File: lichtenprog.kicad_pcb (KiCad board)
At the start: 2 copper layers, 29 x 34 mm, 34 parts, among them J1 USB_B_Mini, J2 Conn_01x08, U1 AMS1117-3.3, U2 CP2102N-A01-GQFN28, U3 MCP6L04x-xSL

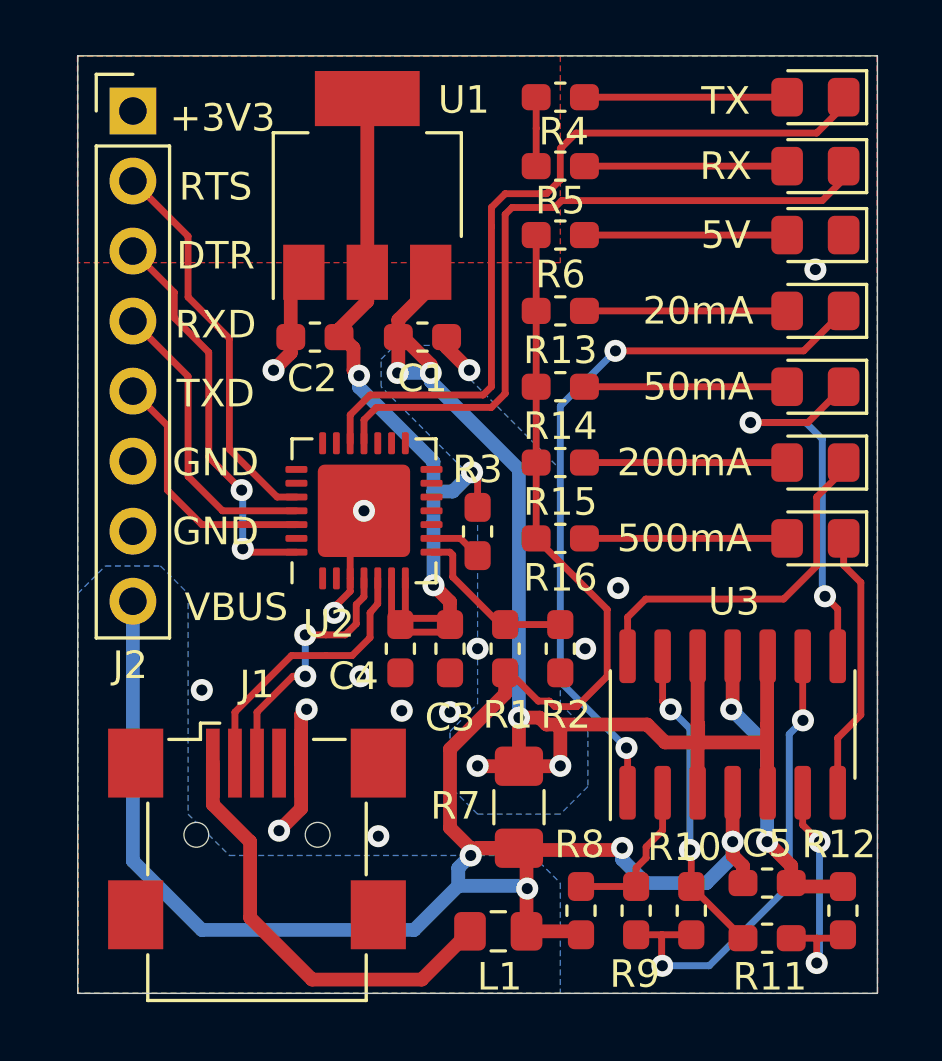
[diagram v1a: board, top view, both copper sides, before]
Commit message: changing pc
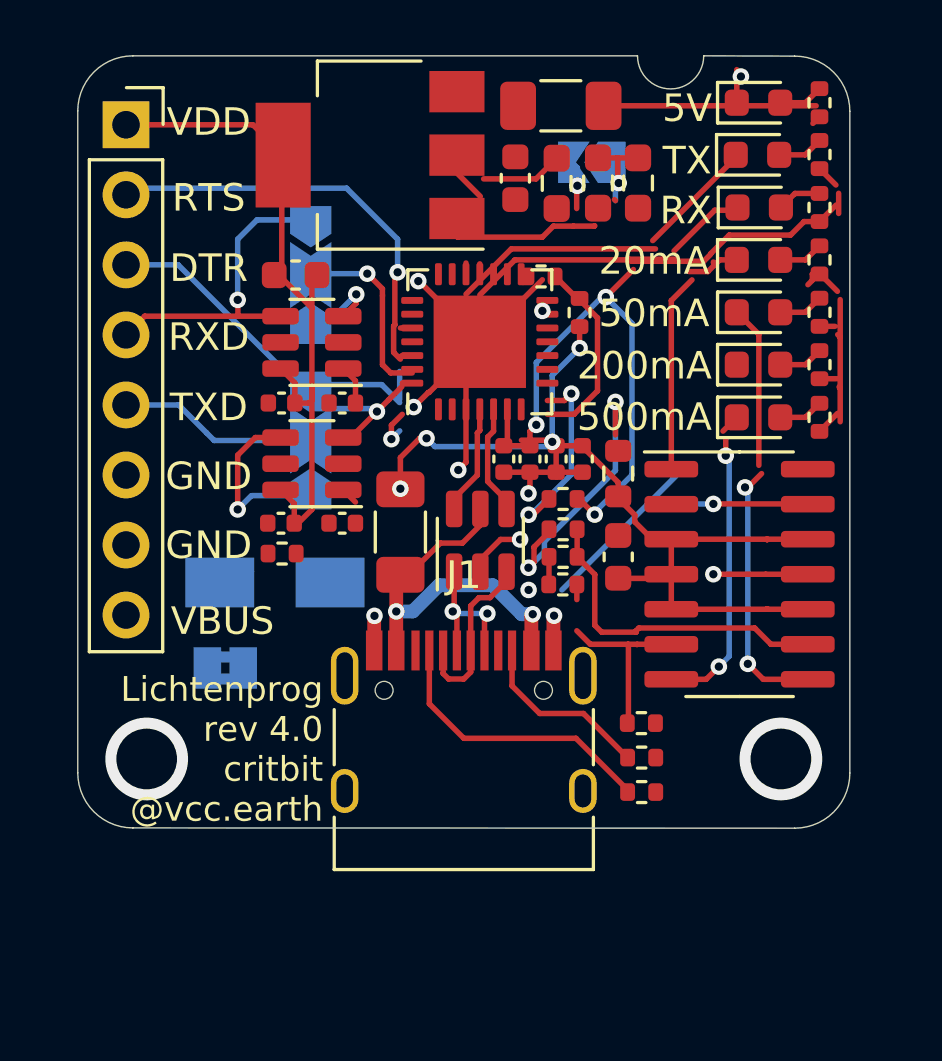
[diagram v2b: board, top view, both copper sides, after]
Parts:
- removed the C1 at (76.5, 56.2)
- removed L1: L_Small, Inductor_SMD:L_0805_2012Metric_Pad1.15x1.40mm_HandSolder
- added C10: 100n, Capacitor_SMD:C_0402_1005Metric, F.Cu at (71.4, 58.6)
- added C11: 100n, Capacitor_SMD:C_0402_1005Metric, F.Cu at (71.4, 63.0)
- added C3: 10u, Capacitor_SMD:C_0603_1608Metric, F.Cu at (71.9, 54.0)
- added C4: 100n, Capacitor_SMD:C_0402_1005Metric, F.Cu at (81.3, 60.6)
- added C5: 2u2, Capacitor_SMD:C_0402_1005Metric, F.Cu at (82.3, 60.6)
- added C8: 100n, Capacitor_SMD:C_0402_1005Metric, F.Cu at (73.6, 58.6)
- added C9: 100n, Capacitor_SMD:C_0402_1005Metric, F.Cu at (73.6, 63.0)
- added D8: 0.8V@100mA, Diode_SMD:D_SMA, B.Cu at (71.2, 65.1)
- added JP1: 1V8_ENA, Jumper:SolderJumper-2_P1.3mm_Open_TrianglePad1.0x1.5mm, B.Cu at (82.6, 49.9)
- added JP2: RX_TRANS_BYPASS, Jumper:SolderJumper-3_P2.0mm_Open_TrianglePad1.0x1.5mm, B.Cu at (72.5, 54.0)
- added JP3: TX_TRANS_BYPASS, Jumper:SolderJumper-3_P2.0mm_Open_TrianglePad1.0x1.5mm, B.Cu at (72.5, 60.0)
- added JP4: LIPO_SIMUL, Jumper:SolderJumper-2_P1.3mm_Bridged2Bar_Pad1.0x1.5mm, B.Cu at (69.3, 68.2)
- added R13: 0R, Resistor_SMD:R_1206_3216Metric_Pad1.30x1.75mm_HandSolder, F.Cu at (75.7, 63.3)
- added R23: DNP/1k, Resistor_SMD:R_0402_1005Metric, F.Cu at (71.4, 64.0)
- added R3: 470, Resistor_SMD:R_0402_1005Metric, F.Cu at (84.5, 72.7)
- added R4: 470, Resistor_SMD:R_0402_1005Metric, F.Cu at (84.5, 71.5)
- added R5: 220, Resistor_SMD:R_0603_1608Metric_Pad0.98x0.95mm_HandSolder, F.Cu at (81.4, 50.6)
- added R6: 270, Resistor_SMD:R_0603_1608Metric_Pad0.98x0.95mm_HandSolder, F.Cu at (82.9, 50.6)
- added R7: 100, Resistor_SMD:R_0603_1608Metric_Pad0.98x0.95mm_HandSolder, F.Cu at (84.3, 50.6)
- added U3: USBLC6-2SC6, Package_TO_SOT_SMD:SOT-23-6, F.Cu at (78.6, 63.6)
- added U5: SN74LVC1T45DBV, Package_TO_SOT_SMD:SOT-23-6, F.Cu at (72.5, 60.8)
- added U6: SN74LVC1T45DBV, Package_TO_SOT_SMD:SOT-23-6, F.Cu at (72.5, 56.4)
- C1: renamed from C5; value 100n -> 2.2u; footprint Capacitor_SMD:C_0603_1608Metric_Pad1.05x0.95mm_HandSolder -> Capacitor_SMD:C_0603_1608Metric
- C2: value 2u2 -> 10u; footprint Capacitor_SMD:C_0603_1608Metric_Pad1.05x0.95mm_HandSolder -> Capacitor_SMD:C_0603_1608Metric
- C6: renamed from C3; footprint Capacitor_SMD:C_0603_1608Metric_Pad1.05x0.95mm_HandSolder -> Capacitor_SMD:C_0402_1005Metric
- C7: renamed from C4; footprint Capacitor_SMD:C_0603_1608Metric_Pad1.05x0.95mm_HandSolder -> Capacitor_SMD:C_0402_1005Metric
- D1: renamed from D3; footprint LED_SMD:LED_0805_2012Metric_Pad1.15x1.40mm_HandSolder -> LED_SMD:LED_0603_1608Metric
- D2: renamed from D4; footprint LED_SMD:LED_0805_2012Metric_Pad1.15x1.40mm_HandSolder -> LED_SMD:LED_0603_1608Metric
- D3: renamed from D5; footprint LED_SMD:LED_0805_2012Metric_Pad1.15x1.40mm_HandSolder -> LED_SMD:LED_0603_1608Metric
- D4: renamed from D6; footprint LED_SMD:LED_0805_2012Metric_Pad1.15x1.40mm_HandSolder -> LED_SMD:LED_0603_1608Metric
- D5: renamed from D1; footprint LED_SMD:LED_0805_2012Metric_Pad1.15x1.40mm_HandSolder -> LED_SMD:LED_0603_1608Metric
- D6: renamed from D7; footprint LED_SMD:LED_0805_2012Metric_Pad1.15x1.40mm_HandSolder -> LED_SMD:LED_0603_1608Metric
- D7: renamed from D2; footprint LED_SMD:LED_0805_2012Metric_Pad1.15x1.40mm_HandSolder -> LED_SMD:LED_0603_1608Metric
- J1: value USB_B_Mini -> USB_C_Receptacle_USB2.0; footprint Connector_USB:USB_Mini-B_Wuerth_65100516121_Horizontal -> Connector_USB:USB_C_Receptacle_HRO_TYPE-C-31-M-12
- J2: value Conn_01x08 -> IO_OUT
- R1: renamed from R6; footprint Resistor_SMD:R_0603_1608Metric_Pad1.05x0.95mm_HandSolder -> Resistor_SMD:R_0402_1005Metric
- R10: footprint Resistor_SMD:R_0603_1608Metric_Pad1.05x0.95mm_HandSolder -> Resistor_SMD:R_0402_1005Metric
- R11: value 3k -> 3.3k; footprint Resistor_SMD:R_0603_1608Metric_Pad1.05x0.95mm_HandSolder -> Resistor_SMD:R_0402_1005Metric
- R12: value 45k -> 47k; footprint Resistor_SMD:R_0603_1608Metric_Pad1.05x0.95mm_HandSolder -> Resistor_SMD:R_0402_1005Metric
- R14: renamed from R1; footprint Resistor_SMD:R_0603_1608Metric_Pad1.05x0.95mm_HandSolder -> Resistor_SMD:R_0402_1005Metric
- R15: renamed from R2; footprint Resistor_SMD:R_0603_1608Metric_Pad1.05x0.95mm_HandSolder -> Resistor_SMD:R_0402_1005Metric
- R16: renamed from R3; footprint Resistor_SMD:R_0603_1608Metric_Pad1.05x0.95mm_HandSolder -> Resistor_SMD:R_0402_1005Metric
- R17: renamed from R13; footprint Resistor_SMD:R_0603_1608Metric_Pad1.05x0.95mm_HandSolder -> Resistor_SMD:R_0402_1005Metric
- R18: renamed from R14; footprint Resistor_SMD:R_0603_1608Metric_Pad1.05x0.95mm_HandSolder -> Resistor_SMD:R_0402_1005Metric
- R19: renamed from R15; footprint Resistor_SMD:R_0603_1608Metric_Pad1.05x0.95mm_HandSolder -> Resistor_SMD:R_0402_1005Metric
- R2: renamed from R7; footprint Resistor_SMD:R_1206_3216Metric_Pad1.42x1.75mm_HandSolder -> Resistor_SMD:R_1206_3216Metric_Pad1.30x1.75mm_HandSolder
- R20: renamed from R4; value 400 -> 470; footprint Resistor_SMD:R_0603_1608Metric_Pad1.05x0.95mm_HandSolder -> Resistor_SMD:R_0402_1005Metric
- R21: renamed from R16; footprint Resistor_SMD:R_0603_1608Metric_Pad1.05x0.95mm_HandSolder -> Resistor_SMD:R_0402_1005Metric
- R22: renamed from R5; value 400 -> 470; footprint Resistor_SMD:R_0603_1608Metric_Pad1.05x0.95mm_HandSolder -> Resistor_SMD:R_0402_1005Metric
- R8: value 100 -> 220; footprint Resistor_SMD:R_0603_1608Metric_Pad1.05x0.95mm_HandSolder -> Resistor_SMD:R_0603_1608Metric
- R9: value 400 -> 330; footprint Resistor_SMD:R_0603_1608Metric_Pad1.05x0.95mm_HandSolder -> Resistor_SMD:R_0402_1005Metric
- U1: value AMS1117-3.3 -> AZ1117-ADJ
- moved R2 25.5 mm to (81.5, 47.8), turned to 180 degrees
- moved R8 15.9 mm to (83.6, 61.1)
- moved R11 14.8 mm to (81.6, 65.2)
- moved R9 14.1 mm to (81.6, 63.2), turned to 0 degrees
- moved R10 13.6 mm to (81.6, 64.2), turned to 180 degrees
- moved R15 13.5 mm to (80.8, 54.0), turned to 180 degrees
- moved C1 13.0 mm to (83.6, 64.2), turned to 90 degrees
- moved R14 12.5 mm to (82.2, 55.3)
- moved R1 10.6 mm to (90.9, 47.7), turned to -90 degrees
- moved R21 10.4 mm to (90.9, 59.1), turned to -90 degrees
- moved R19 10.0 mm to (90.9, 57.2), turned to -90 degrees
- moved R12 9.98 mm to (84.4, 70.2), turned to 0 degrees
- moved R18 9.78 mm to (90.9, 55.3), turned to -90 degrees
- moved R20 9.63 mm to (90.9, 49.6), turned to 90 degrees
- moved R17 9.58 mm to (90.9, 53.4), turned to -90 degrees
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- renumbered U3 to U2, U2 to U4
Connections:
- C2 pad 1: +3V3 -> Net-(C2-Pad1)
- J2 pad 1: +3V3 -> VDD
- J2 pad 4: /PROG_RXD -> /PROG_RX_VDD
- J2 pad 5: /PROG_TXD -> /PROG_TX_VDD
- J2 pad 8: VBUS -> Net-(D8-Pad1)
- R2 pad 2: Net-(C1-Pad1) -> Net-(C2-Pad1)
- U1 pad 1: GND -> Net-(JP1-Pad2)
- U1 pad 2: +3V3 -> VDD
- U1 pad 3: Net-(C1-Pad1) -> Net-(C2-Pad1)
- U2 pad 10: Net-(C1-Pad1) -> VBUS
- U2 pad 12: Net-(C1-Pad1) -> VBUS
- U2 pad 3: Net-(C1-Pad1) -> VBUS
- U2 pad 5: Net-(C1-Pad1) -> VBUS
- U4 pad 1: Net-(U2-Pad1) -> unconnected-(U4-Pad1)
- U4 pad 10: Net-(U2-Pad10) -> unconnected-(U4-Pad10)
- U4 pad 11: Net-(U2-Pad11) -> unconnected-(U4-Pad11)
- U4 pad 12: Net-(U2-Pad12) -> unconnected-(U4-Pad12)
- U4 pad 13: Net-(U2-Pad13) -> unconnected-(U4-Pad13)
- U4 pad 14: Net-(U2-Pad14) -> unconnected-(U4-Pad14)
- U4 pad 15: Net-(U2-Pad15) -> unconnected-(U4-Pad15)
- U4 pad 16: Net-(U2-Pad16) -> unconnected-(U4-Pad16)
- U4 pad 17: Net-(U2-Pad17) -> unconnected-(U4-Pad17)
- U4 pad 2: Net-(U2-Pad2) -> unconnected-(U4-Pad2)
- U4 pad 20: Net-(U2-Pad20) -> unconnected-(U4-Pad20)
- U4 pad 21: Net-(U2-Pad21) -> unconnected-(U4-Pad21)
- U4 pad 22: Net-(U2-Pad22) -> unconnected-(U4-Pad22)
- U4 pad 23: Net-(U2-Pad23) -> unconnected-(U4-Pad23)
- U4 pad 25: /PROG_RXD -> /PROG_RX_3V3
- U4 pad 26: /PROG_TXD -> /PROG_TX_3V3
- U4 pad 27: Net-(U2-Pad27) -> unconnected-(U4-Pad27)
- U4 pad 4: Net-(J1-Pad3) -> Net-(U3-Pad6)
- U4 pad 5: Net-(J1-Pad2) -> Net-(U3-Pad4)
- U4 pad 7: +3V3 -> VBUS
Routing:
- net Net-(C1-Pad1): track 47.8 -> 0.00 mm, vias 5 -> 0
- net VBUS: track 78.0 -> 43.7 mm
- net VDD: track 0.00 -> 29.6 mm
- net /PROG_TX_3V3: track 0.00 -> 20.2 mm, vias 0 -> 2
- net Net-(D2-Pad1): track 26.7 -> 9.10 mm, vias 2 -> 0
- net Net-(D5-Pad1): track 28.4 -> 12.2 mm
- net Net-(J1-Pad1): track 15.8 -> 0.00 mm
- net Net-(D7-Pad1): track 26.1 -> 11.0 mm
- net /DTR: track 14.4 -> 0.36 mm, vias 2 -> 0
- net Net-(J1-PadA4): track 0.00 -> 14.0 mm, vias 0 -> 2
- net Net-(D4-Pad1): track 13.2 -> 0.00 mm
- net /PROG_RX_VDD: track 0.00 -> 11.6 mm, vias 0 -> 1
- net /PROG_RXD: track 10.9 -> 0.00 mm
- net Net-(J1-PadA5): track 0.00 -> 10.5 mm
- net Net-(J1-Pad2): track 10.1 -> 0.00 mm
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- removed copper zone on F.Cu, net +3V3
- removed copper zone on B.Cu, net GND
- removed copper zone on F.Cu, net GND
- removed copper zone on B.Cu, net Net-(C1-Pad1)
- removed copper zone on B.Cu, net VBUS
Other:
- board size 29 x 34 mm -> 28 x 28 mm
- net class Default removed
- board text added: "3V3"
- board text added: "Lichtenprog rev 4.0 critbit @vcc.earth"
- board text added: "VDD"
- board text removed: "+3V3"
- board text removed: "Lichtenprog rev 2.0"
